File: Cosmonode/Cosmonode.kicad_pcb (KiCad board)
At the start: 2 copper layers, 47 x 34.3 mm, 51 parts, among them J1 CONN_01X12, J10 WEEE_Logo, J11 Aloes_Logo, J12 Aloes_mini_Logo, J13 CONN_01X05, J14 GS2, J2 CONN_01X12, J3 GS2, J4 OSHW, J5 CONN_01X02, J8 USB_OTG, J9 GS2, P1 COAX, Q1 BSS123, SW1 SW_DIP_x01, U1 ATMEGA328P-AU, U3 RN2483, U4 M25P40, U5 XC6206P332MR, U6 ATSHA204, U7 MCP73811T-420I/OT, Y1 Crystal_GND2

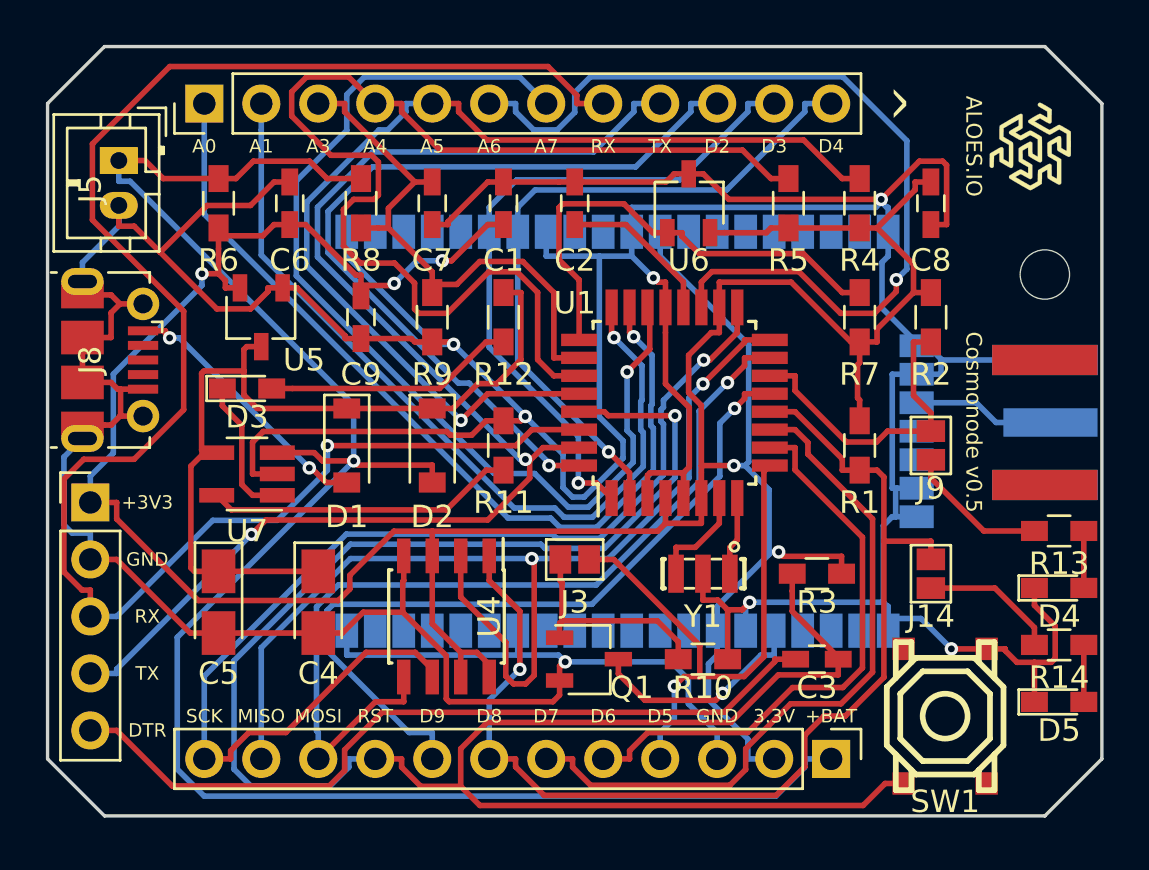
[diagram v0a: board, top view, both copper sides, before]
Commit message: update to V0.7 (WIP)
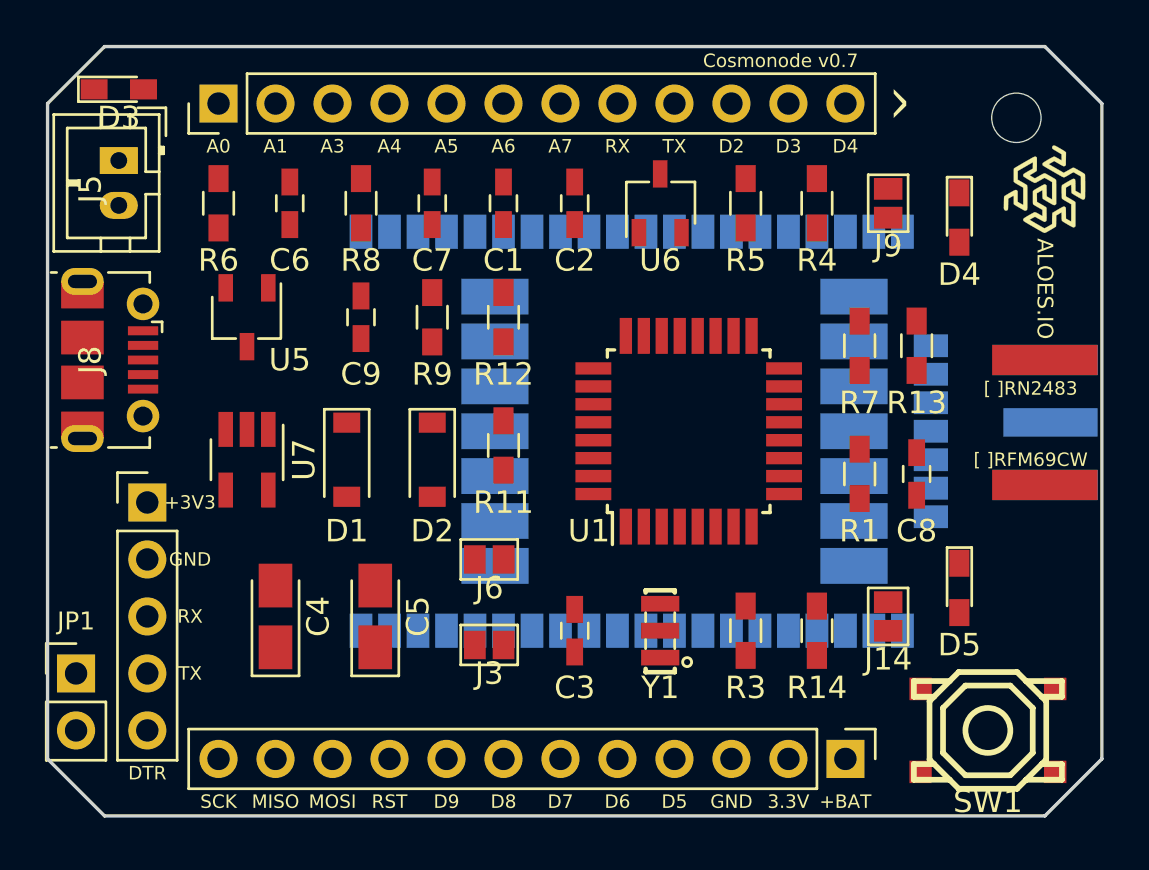
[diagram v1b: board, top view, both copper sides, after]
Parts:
- removed Q1: BSS123, TO_SOT_Packages_SMD:TSOT-23
- removed R10, R2: 10k, Resistors_SMD:R_0603_HandSoldering
- removed U4: M25P40, Housings_SOIC:SOIC-8_3.9x4.9mm_Pitch1.27mm
- added J6: GS2, Connectors:GS2, F.Cu at (165.7, 100.3)
- added JP1: Jumper_NO_Small, Pin_Headers:Pin_Header_Straight_1x02_Pitch2.54mm, F.Cu at (147.3, 105.4)
- added U2: RFM69CW, w_rf_modules:RFM12B_SMD, B.Cu at (174.0, 94.6)
- moved J10 39.3 mm to (154.9, 88.3)
- moved D4 17.1 mm to (186.7, 85.1), turned to 270 degrees
- moved D3 14.5 mm to (149.2, 79.4)
- moved C8 12.1 mm to (184.8, 96.5)
- moved J9 11.0 mm to (183.5, 84.5)
- moved C3 10.9 mm to (169.5, 103.5), turned to 270 degrees
- moved R14 10.8 mm to (180.3, 103.5), turned to 90 degrees
- moved R13 10.4 mm to (184.8, 90.8), turned to 270 degrees
- moved MK1 7.10 mm to (189.2, 80.6)
- moved C5 7.01 mm to (160.7, 102.9), turned to 90 degrees
- moved D5 6.75 mm to (186.7, 101.6), turned to 270 degrees
- moved J3 5.39 mm to (165.7, 104.1), turned to 270 degrees
- moved R3 4.07 mm to (177.2, 103.5), turned to 90 degrees
- moved J11 3.86 mm to (188.0, 86.4)
- moved Y1 3.17 mm to (173.4, 103.5), turned to 90 degrees
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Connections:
- net Net-(P1-Pad1) renamed ANT
- net SCK renamed D13/SCK
- D1 pad 1: Net-(C4-Pad1) -> Net-(D1-Pad1)
- D2 pad 1: Net-(C4-Pad1) -> Net-(D1-Pad1)
- J14 pad 2: D8 -> A7
- J2 pad 10: MOSI -> D11/MOSI
- J2 pad 11: MISO -> D12/MISO
- J3 pad 1: Net-(J3-Pad1) -> /RADIO_RESET
- J3 pad 2: D5 -> D12/MISO
- J9 pad 2: D10 -> A6
- P1 pad 3: GND -> (no net)
- P1 pad 4: GND -> (no net)
- P1 pad 5: GND -> (no net)
- R12 pad 2: Net-(C4-Pad1) -> Net-(D1-Pad1)
- U1 pad 15: MOSI -> D11/MOSI
- U1 pad 16: MISO -> D12/MISO
- U3 pad 6: D3 -> D11/MOSI
- U3 pad 7: D4 -> D10
- U7 pad 4: Net-(C4-Pad1) -> Net-(D1-Pad1)
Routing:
- net GND: track 268.2 -> 0.00 mm, vias 7 -> 0
- net +3V3: track 150.2 -> 0.00 mm, vias 5 -> 0
- net RST: track 92.7 -> 0.00 mm, vias 1 -> 0
- net +BATT: track 85.2 -> 0.00 mm, vias 1 -> 0
- net RX: track 77.9 -> 0.00 mm, vias 1 -> 0
- net TX: track 59.4 -> 0.00 mm, vias 2 -> 0
- net A4: track 52.1 -> 0.00 mm
- net D13/SCK: track 50.1 -> 0.00 mm, vias 1 -> 0
- net D8: track 50.1 -> 0.00 mm, vias 1 -> 0
- net MISO: track 48.5 -> 0.00 mm, vias 2 -> 0
- net A5: track 46.6 -> 0.00 mm, vias 1 -> 0
- net A7: track 46.3 -> 0.00 mm, vias 1 -> 0
- net A6: track 40.1 -> 0.00 mm, vias 1 -> 0
- net MOSI: track 39.6 -> 0.00 mm, vias 1 -> 0
- net A0: track 39.5 -> 0.00 mm, vias 1 -> 0
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- removed copper zone on B.Cu, net GND
- removed copper zone on F.Cu, net GND
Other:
- board text added: "Cosmonode v0.7"
- board text added: "[ ]RFM69CW"
- board text added: "[ ]RN2483"
- board text removed: "Cosmonode v0.5"
- board text removed: "Cosmonode v0.5, by Getlarge https://aloes.io"
